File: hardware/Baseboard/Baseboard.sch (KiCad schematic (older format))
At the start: 0 parts

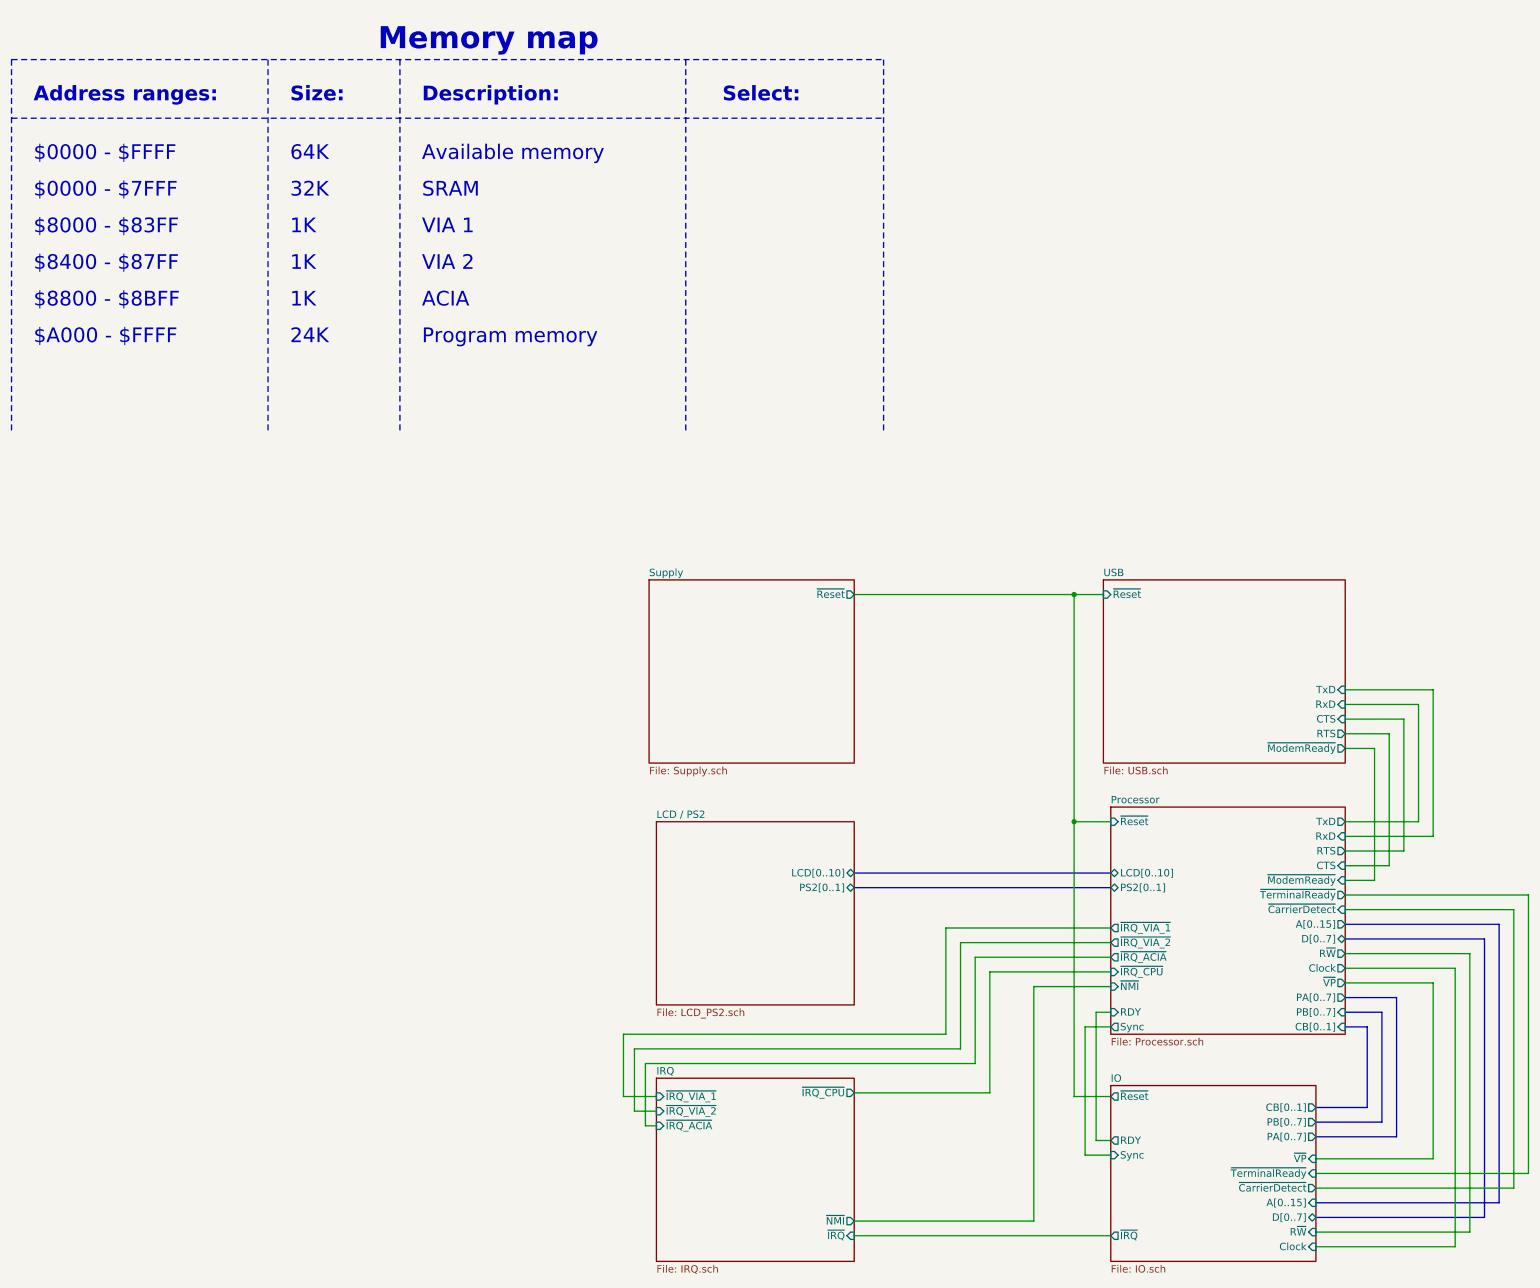
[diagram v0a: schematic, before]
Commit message: Working on PCB
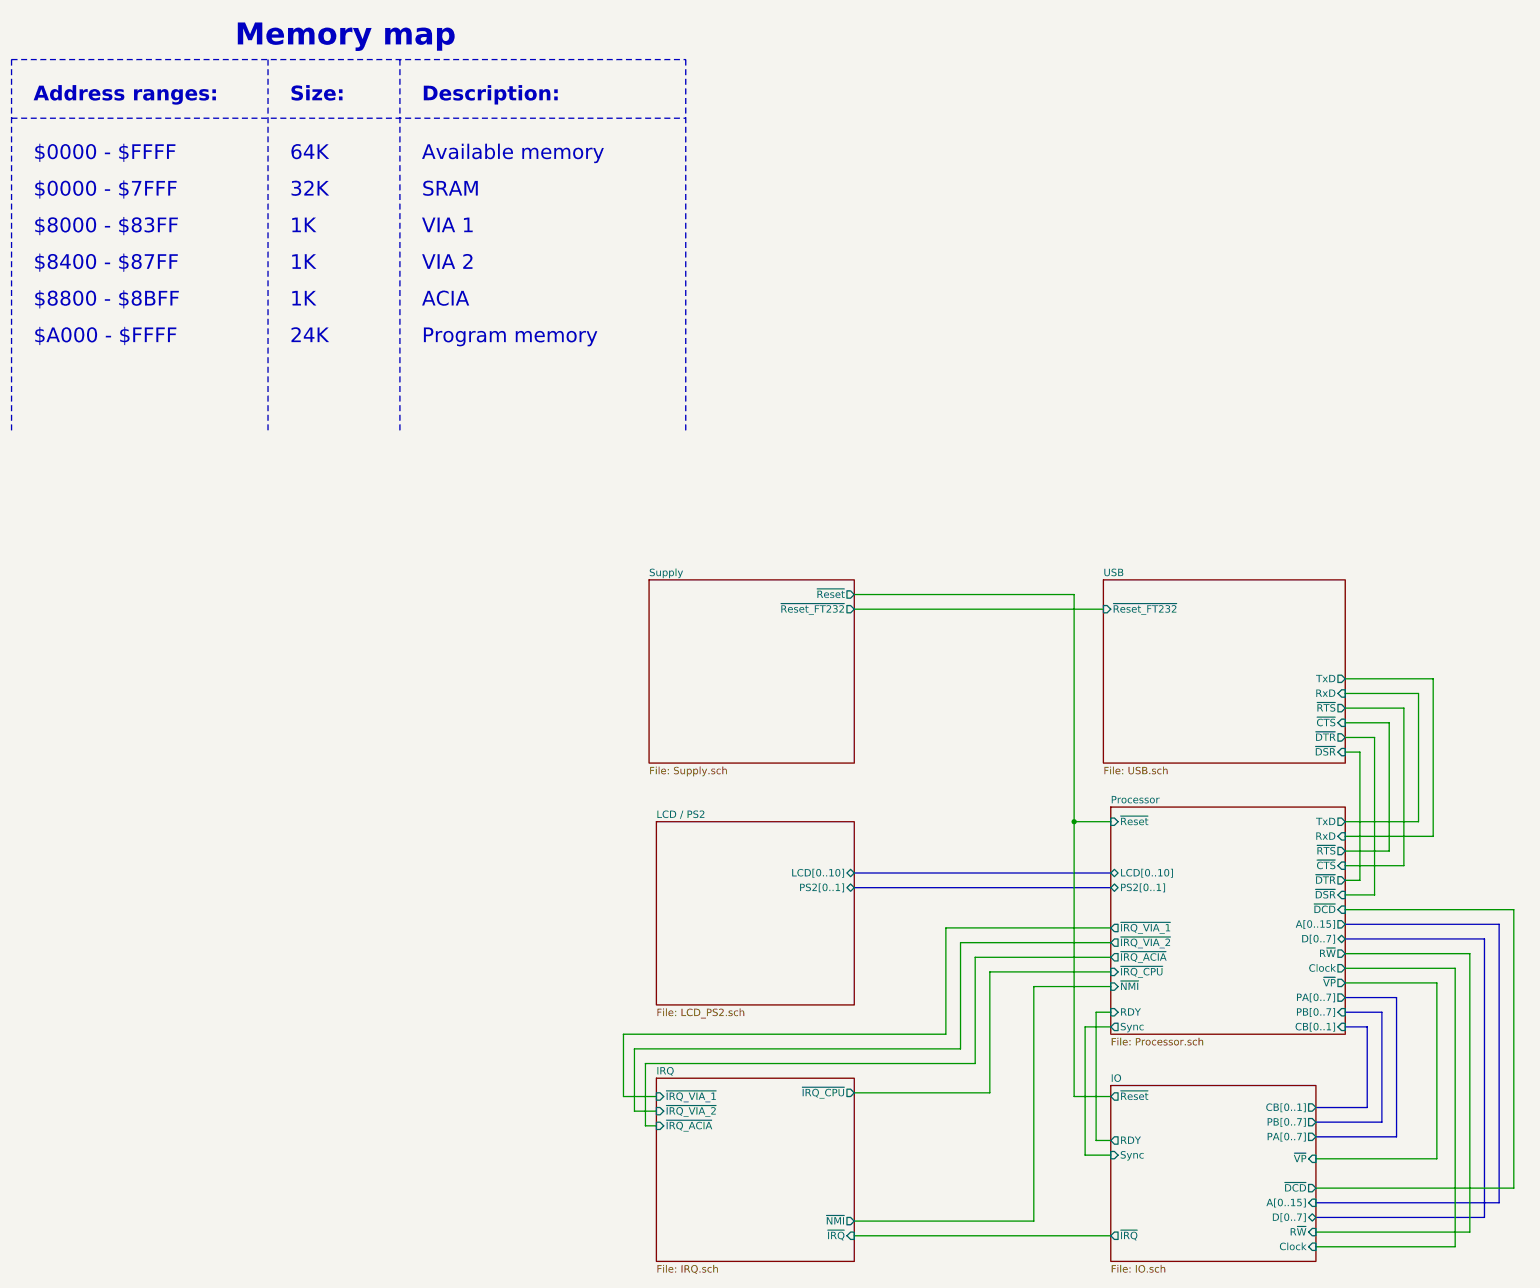
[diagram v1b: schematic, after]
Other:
- note removed: "Select:"
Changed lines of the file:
@@
 Sheet 1 7
 Title "Baseboard"
-Date "2019-11-24"
-Rev "1.1"
+Date "2020-01-17"
+Rev "1.0"
 Comp "https://www.kampis-elektroecke.de"
 Comment1 "Author: Daniel Kampert"
@@
 Text Notes 3550 2100 0    100  ~ 0
 SRAM
-Text Notes 5600 1450 0    100  ~ 20
-Select:
 Wire Notes Line width 18 style solid
 	5350 1150 5350 3700
-Text Notes 3250 1100 0    150  ~ 30
+Text Notes 2275 1075 0    150  ~ 30
 Memory map
 $Sheet
@@
 F1 "Supply.sch" 50
 F2 "~Reset" O R 6500 4800 50
+F3 "~Reset_FT232" O R 6500 4900 50
 $EndSheet
 Wire Bus Line
@@
 F5 "R~W" I R 9650 9150 50
 F6 "Clock" I R 9650 9250 50
-F7 "~TerminalReady" I R 9650 8750 50
-F8 "~CarrierDetect" O R 9650 8850 50
-F9 "~Reset" O L 8250 8225 50
-F10 "CB[0..1]" O R 9650 8300 50
-F11 "A[0..15]" I R 9650 8950 50
-F12 "D[0..7]" B R 9650 9050 50
-F13 "RDY" O L 8250 8525 50
-F14 "Sync" I L 8250 8625 50
-F15 "~VP" I R 9650 8650 50
+F7 "~Reset" O L 8250 8225 50
+F8 "CB[0..1]" O R 9650 8300 50
+F9 "A[0..15]" I R 9650 8950 50
+F10 "D[0..7]" B R 9650 9050 50
+F11 "RDY" O L 8250 8525 50
+F12 "Sync" I L 8250 8625 50
+F13 "~VP" I R 9650 8650 50
+F14 "~DCD" O R 9650 8850 50
 $EndSheet
 Text Notes 900  1850 0    100  ~ 0
 $0000 - $FFFF\n
 Wire Notes Line width 18 style solid
-	750  1550 6700 1550
-Wire Notes Line width 18 style solid
-	750  1150 6700 1150
-Wire Notes Line width 18 style solid
-	6700 1150 6700 3700
+	750  1550 5350 1550
+Wire Notes Line width 18 style solid
+	750  1150 5350 1150
 Wire Notes Line width 18 style solid
 	750  1150 750  3700
 Wire Wire Line
-	9850 5450 10450 5450
-Wire Wire Line
-	10350 5550 9850 5550
-Wire Wire Line
-	9850 5650 10250 5650
-Wire Wire Line
-	10250 5650 10250 6550
-Wire Wire Line
-	10250 6550 9850 6550
-Wire Wire Line
-	10150 5750 9850 5750
-Wire Wire Line
-	9850 5850 10050 5850
-Wire Wire Line
-	10050 5850 10050 6750
-Wire Wire Line
-	10050 6750 9850 6750
+	9850 5375 10450 5375
+Wire Wire Line
+	10350 5475 9850 5475
+Wire Wire Line
+	9850 5575 10250 5575
+Wire Wire Line
+	10150 6550 9850 6550
+Wire Wire Line
+	9850 5775 10050 5775
 Wire Wire Line
 	9850 6350 10350 6350
 Wire Wire Line
-	10350 6350 10350 5550
+	10350 6350 10350 5475
 Wire Wire Line
 	9850 6450 10450 6450
@@
 24K
 Wire Wire Line
-	10450 5450 10450 6450
+	10450 5375 10450 6450
 $Sheet
 S 5150 6350 1350 1250
@@
 F4 "TxD" O R 9850 6350 50
 F5 "RxD" I R 9850 6450 50
-F6 "RTS" O R 9850 6550 50
-F7 "CTS" I R 9850 6650 50
-F8 "~NMI" I L 8250 7475 50
-F9 "R~W" O R 9850 7250 50
-F10 "LCD[0..10]" B L 8250 6700 50
-F11 "PS2[0..1]" B L 8250 6800 50
-F12 "~ModemReady" I R 9850 6750 50
-F13 "Clock" O R 9850 7350 50
-F14 "~TerminalReady" O R 9850 6850 50
-F15 "~CarrierDetect" I R 9850 6950 50
-F16 "~Reset" I L 8250 6350 50
-F17 "~IRQ_VIA_2" O L 8250 7175 50
-F18 "~IRQ_VIA_1" O L 8250 7075 50
-F19 "~IRQ_ACIA" O L 8250 7275 50
-F20 "~IRQ_CPU" I L 8250 7375 50
-F21 "CB[0..1]" I R 9850 7750 50
-F22 "A[0..15]" O R 9850 7050 50
-F23 "D[0..7]" B R 9850 7150 50
-F24 "RDY" I L 8250 7650 50
-F25 "Sync" O L 8250 7750 50
-F26 "~VP" O R 9850 7450 50
+F6 "~NMI" I L 8250 7475 50
+F7 "R~W" O R 9850 7250 50
+F8 "LCD[0..10]" B L 8250 6700 50
+F9 "PS2[0..1]" B L 8250 6800 50
+F10 "Clock" O R 9850 7350 50
+F11 "~Reset" I L 8250 6350 50
+F12 "~IRQ_VIA_2" O L 8250 7175 50
+F13 "~IRQ_VIA_1" O L 8250 7075 50
+F14 "~IRQ_ACIA" O L 8250 7275 50
+F15 "~IRQ_CPU" I L 8250 7375 50
+F16 "CB[0..1]" I R 9850 7750 50
+F17 "A[0..15]" O R 9850 7050 50
+F18 "D[0..7]" B R 9850 7150 50
+F19 "RDY" I L 8250 7650 50
+F20 "Sync" O L 8250 7750 50
+F21 "~VP" O R 9850 7450 50
+F22 "~RTS" O R 9850 6550 50
+F23 "~CTS" I R 9850 6650 50
+F24 "~DSR" I R 9850 6850 50
+F25 "~DTR" O R 9850 6750 50
+F26 "~DCD" I R 9850 6950 50
 $EndSheet
 Wire Bus Line
@@
 	8250 6700 6500 6700
 Wire Wire Line
-	10150 6650 10150 5750
-Wire Wire Line
-	9850 6650 10150 6650
-$Sheet
-S 8200 4700 1650 1250
-U 5E9064F2
-F0 "USB" 50
-F1 "USB.sch" 50
-F2 "TxD" I R 9850 5450 50
-F3 "RxD" I R 9850 5550 50
-F4 "CTS" I R 9850 5650 50
-F5 "RTS" O R 9850 5750 50
-F6 "~ModemReady" O R 9850 5850 50
-F7 "~Reset" I L 8200 4800 50
-$EndSheet
-Wire Wire Line
 	10600 7350 10600 9250
 Wire Bus Line
@@
 Wire Bus Line
 	10200 8500 10200 7550
-Wire Wire Line
-	11100 6850 11100 8750
-Wire Wire Line
-	9850 6850 11100 6850
-Wire Wire Line
-	9650 8750 11100 8750
-Wire Wire Line
-	9650 8850 11000 8850
-Wire Wire Line
-	11000 8850 11000 6950
-Wire Wire Line
-	11000 6950 9850 6950
 $Sheet
 S 5150 8100 1350 1250
@@
 Wire Wire Line
 	8000 4800 8000 6350
-Connection ~ 8000 4800
-Wire Wire Line
-	8000 4800 8200 4800
-Wire Wire Line
-	9850 7450 10450 7450
-Wire Wire Line
-	10450 7450 10450 8650
-Wire Wire Line
-	10450 8650 9650 8650
+Wire Wire Line
+	9850 7450 10475 7450
+Wire Wire Line
+	10475 7450 10475 8650
+Wire Wire Line
+	10475 8650 9650 8650
+$Sheet
+S 8200 4700 1650 1250
+U 5E9064F2
+F0 "USB" 50
+F1 "USB.sch" 50
+F2 "RxD" I R 9850 5475 50
+F3 "~CTS" I R 9850 5675 50
+F4 "~RTS" O R 9850 5575 50
+F5 "~DTR" O R 9850 5775 50
+F6 "~DSR" I R 9850 5875 50
+F7 "TxD" O R 9850 5375 50
+F8 "~Reset_FT232" I L 8200 4900 50
+$EndSheet
+Wire Wire Line
+	9850 5875 9950 5875
+Wire Wire Line
+	9950 5875 9950 6750
+Wire Wire Line
+	9850 6950 11000 6950
+Wire Wire Line
+	11000 6950 11000 8850
+Wire Wire Line
+	11000 8850 9650 8850
+Wire Wire Line
+	10150 5675 10150 6550
+Wire Wire Line
+	9850 5675 10150 5675
+Wire Wire Line
+	10250 5575 10250 6650
+Wire Wire Line
+	9850 6650 10250 6650
+Wire Wire Line
+	10050 5775 10050 6850
+Wire Wire Line
+	9850 6750 9950 6750
+Wire Wire Line
+	9850 6850 10050 6850
+Wire Wire Line
+	6500 4900 8200 4900
 $EndSCHEMATC
